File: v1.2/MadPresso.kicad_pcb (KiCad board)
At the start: 2 copper layers, 108 x 57.5 mm, 76 parts, among them J1 Conn_01x07, J2 Conn_01x03, J3 Conn_01x02, J4 Conn_01x04, Q1 BC847, Q2 BSS84, Q3 T835-600B, Q4 2N7002, Q5 T835-600B, Q6 2N7002, Q7 T835-600B, Q8 2N7002, U1 LTV-356T, U2 ADC101C021CIMK, U3 WeMos_D1_mini, U4 MID400, U5 MID400, U6 TLP160G, U7 TLP160G, U8 TLP160G

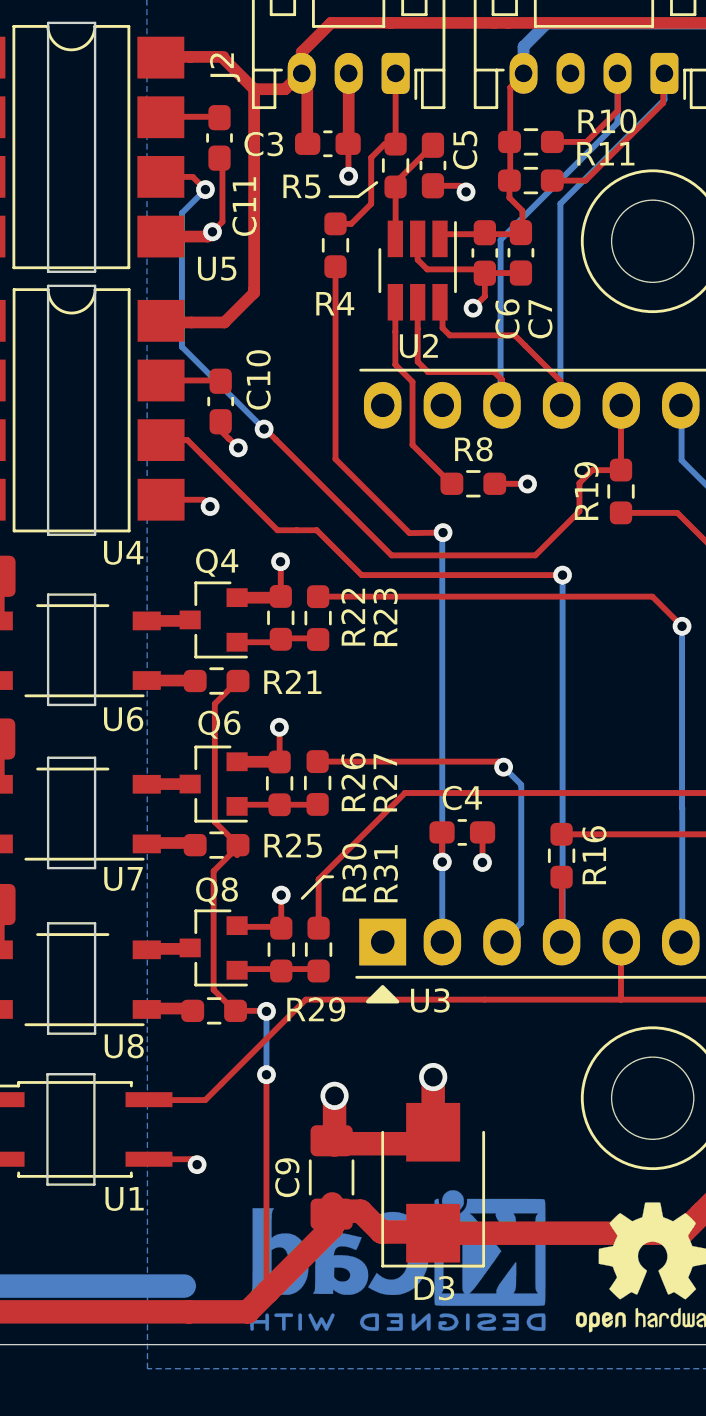
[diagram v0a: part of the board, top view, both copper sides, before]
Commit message: some minor details
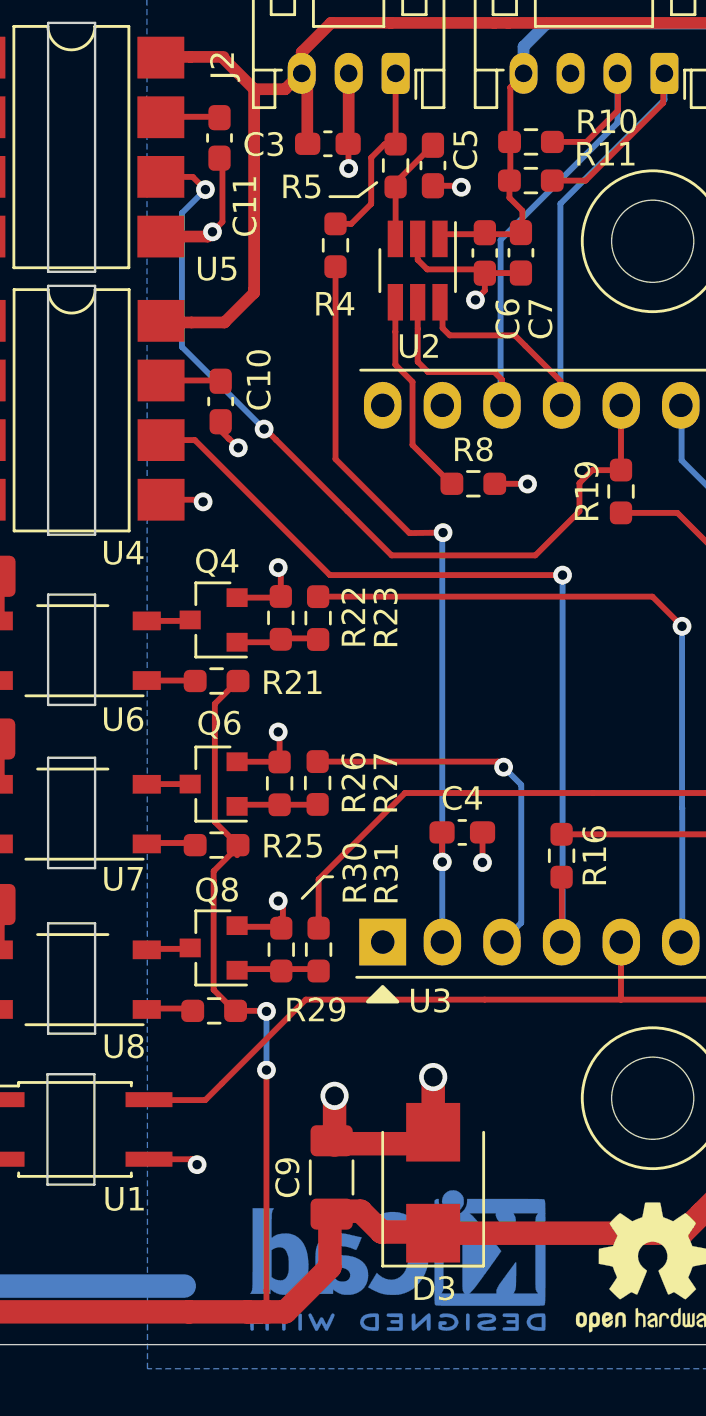
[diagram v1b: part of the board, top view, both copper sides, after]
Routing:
- net GND: track 85.1 -> 83.0 mm
- net +5V: track 182.1 -> 183.3 mm
